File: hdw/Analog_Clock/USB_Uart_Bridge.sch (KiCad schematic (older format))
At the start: 37 parts, among them J1301 USB_B_Mini, U1301 74LVC1G07, U1302 74LVC1G07, U1303 TLV6700, U1304 FT234XD, U1305 TPD3S014DBVR

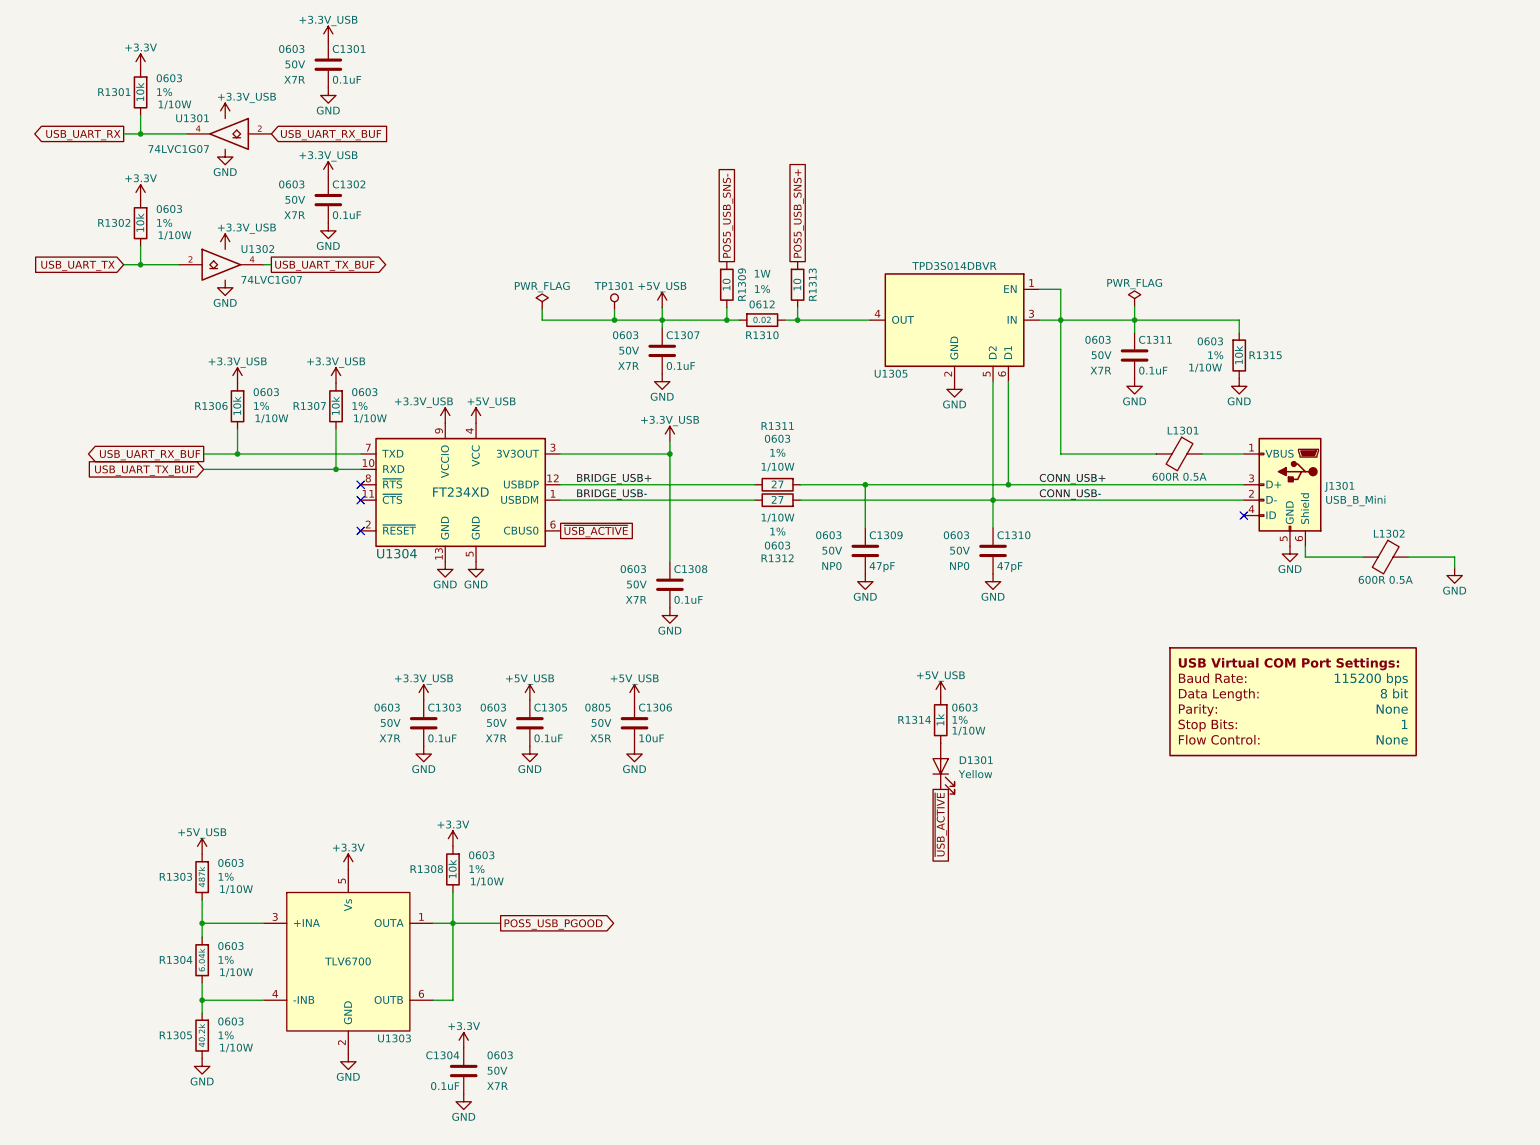
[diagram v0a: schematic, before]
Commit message: Much more schematic progress
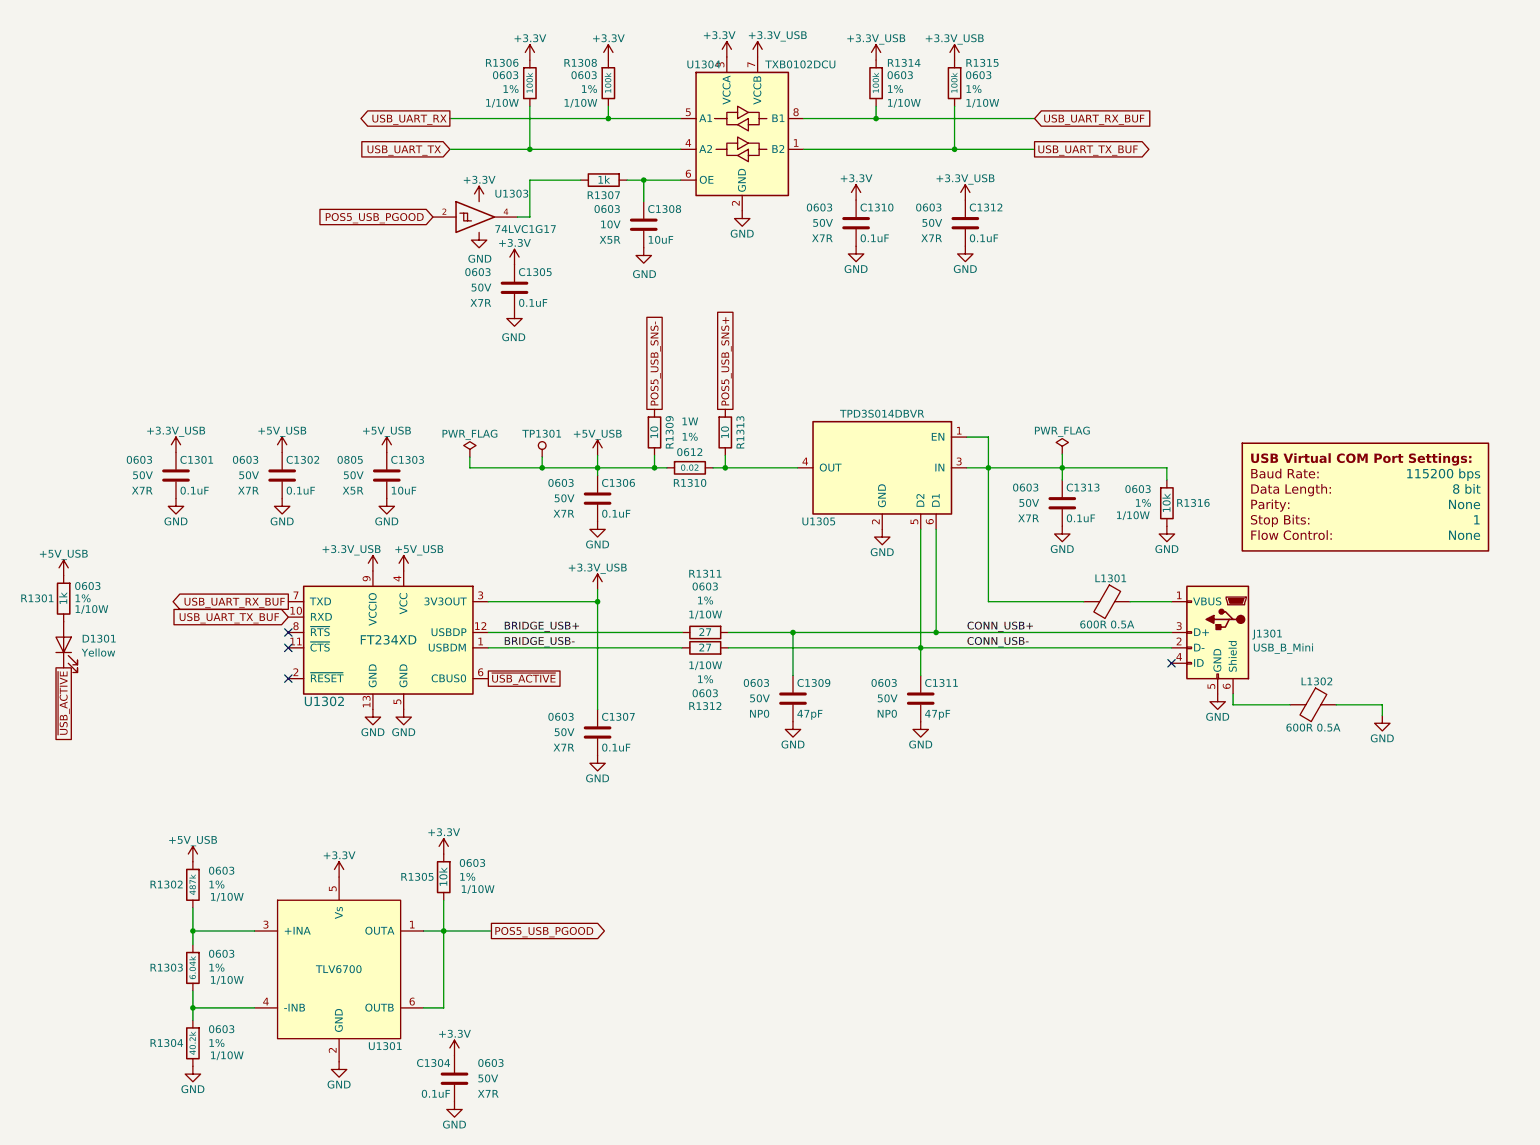
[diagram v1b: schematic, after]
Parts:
- removed C1301, C1302: 0.1uF, Capacitors_SMD:C_0603, symbol Custom_Library:C_Custom
- removed R1301, R1302: 10k, Resistors_SMD:R_0603, symbol Custom_Library:R_Custom
- removed U1301, U1302: 74LVC1G07, TO_SOT_Packages_SMD:SOT-353_SC-70-5, symbol Custom_Library:74LVC1G07_Power
- added C1305, C1310, C1312: 0.1uF, Capacitors_SMD:C_0603, symbol Custom_Library:C_Custom
- added C1308: 10uF, Capacitors_SMD:C_0603, symbol Custom_Library:C_Custom
- added R1308, R1314, R1315: 100k, Resistors_SMD:R_0603, symbol Custom_Library:R_Custom
- added U1303: 74LVC1G17, TO_SOT_Packages_SMD:SOT-353_SC-70-5, symbol Custom_Library:74LVC1G17_Power
- added U1304: TXB0102DCU, Package_SO:VSSOP-8_2.4x2.1mm_P0.5mm, symbol Logic_LevelTranslator:TXB0102DCU
- R1301: renamed from R1314; Digi-Key PN (none) -> 311-1.00KHRCT-ND
- R1302: renamed from R1303; Digi-Key PN (none) -> 311-487KHRCT-ND
- R1303: renamed from R1304; Digi-Key PN (none) -> RMCF0603FT6K04CT-ND
- R1304: renamed from R1305; Digi-Key PN (none) -> RMCF0603FT40K2CT-ND
- R1305: renamed from R1308; Digi-Key PN (none) -> YAG2321CT-ND
- R1306: value 10k -> 100k; Digi-Key PN (none) -> RMCF0603FT100KCT-ND
- R1307: value 10k -> 1k; Digi-Key PN (none) -> 311-1.00KHRCT-ND
- R1309, R1313: Digi-Key PN (none) -> YAG2321CT-ND
- R1311, R1312: Digi-Key PN (none) -> 311-27.0HRCT-ND
- R1316: renamed from R1315; Digi-Key PN (none) -> YAG2321CT-ND
- renumbered C1303 to C1301, C1305 to C1302, C1306 to C1303, C1307 to C1306, C1308 to C1307, C1310 to C1311, C1311 to C1313, U1303 to U1301, U1304 to U1302
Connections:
- net +3.3V_USB: now also C1312.1, R1314.1, R1315.1, U1304.7 (VCCB); no longer R1306.1, R1307.1
- net +3V3: now also R1306.1, C1305.1, C1310.1, R1308.1, U1303.5 (VCC), U1304.3 (VCCA)
- net GND: now also C1305.2, C1308.2, C1310.2, C1312.2, U1303.3 (GND), U1304.2 (GND)
- net POS5_USB_PGOOD: now also U1303.2
- net USB_UART_RX: now also R1308.2, U1304.5 (A1)
- net USB_UART_RX_BUF: now also R1314.2, U1304.8 (B1); no longer R1306.2
- net USB_UART_TX: now also R1306.2, U1304.4 (A2)
- net USB_UART_TX_BUF: now also R1315.2, U1304.1 (B2); no longer R1307.2
- new net: C1308.1, R1307.1, U1304.6 (OE)
- new net: R1307.2, U1303.4
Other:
- moved on the sheet: C1301, C1302, C1303, C1304, C1306, C1307, C1309, C1311, C1313, D1301, J1301, L1301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
